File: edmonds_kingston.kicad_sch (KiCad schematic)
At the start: 22 parts

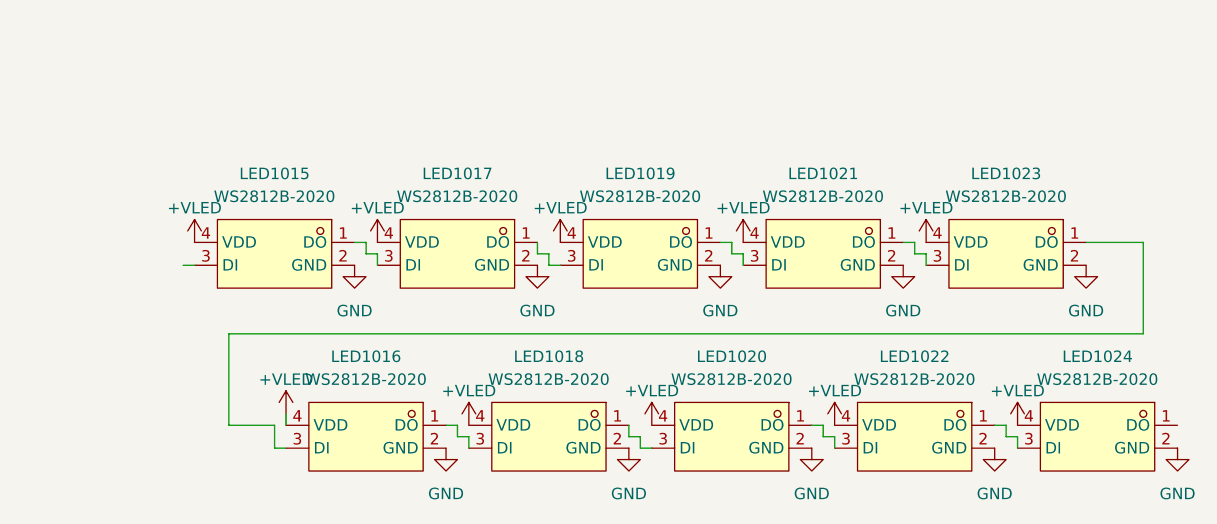
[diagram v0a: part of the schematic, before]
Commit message: single ferry track checkpoint
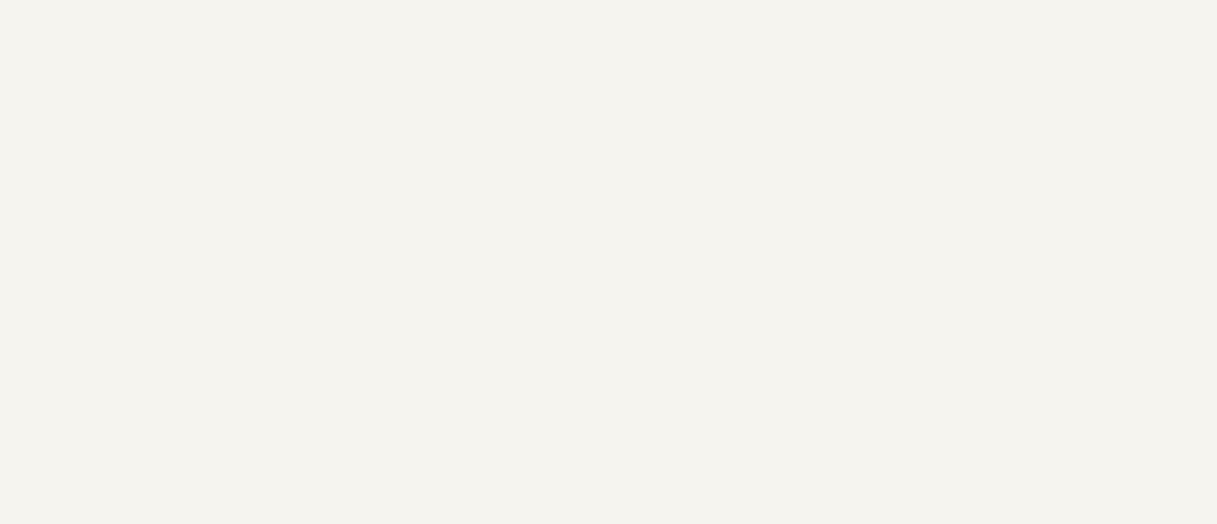
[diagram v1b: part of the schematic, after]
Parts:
- removed LED1015, LED1016, LED1017, LED1018, LED1019, LED1020, LED1021, LED1022, LED1023, LED1024: WS2812B-2020, EasyEDA:LED-SMD_4P-L2.0-W2.0-TL_WS2812B-2020, symbol EasyEDA:WS2812B-2020
